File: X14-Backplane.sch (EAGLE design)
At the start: 34 parts, among them J2 PXC-PTSM-04-RA-1778641, J3 PXC-8-RA-1778683, J8 PXC-8-RA-1778683

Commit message: STEPS!
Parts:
- DIST_TO_BACKPLANE: device Samtec MPPT Hermaphoditic 10 pos - MPPT-10-01-01-L-RA-SD:MPPT-10-01-01-L-RA-SD -> CONN, Samtec MPPT Hermaphoditic 10 pos - MPPT-10-01-01-L-RA-SD:MPPT-10-01-01-L-RA-SD
- J2: device Phoenix Contact PTSM-04-V-1778573:PXC-PTSM-04-RA-1778641 -> CONN, Phoenix Contact PTSM-04-V-1778573:PXC-PTSM-04-RA-1778641
- J3, J8: device Phoenix Contact PTSM 8 pin:PXC-8-RA-1778683 -> CONN, Phoenix Contact PTSM 8 pin:PXC-8-RA-1778683
- U$1, U$2, U$3: device BLHeli_32 45A:BACKPLANE_CONNECTORSBKP -> Conn, Backplane-ESC-Controller:BACKPLANE_CONNECTORSBKP
- U$5, U$6, U$7: device Backplane_ESC_adapter:BACKPLANE_ESC_ADAPTER_PWRBKP -> CONN, Backplane_ESC_adapter:BACKPLANE_ESC_ADAPTER_PWRBKP
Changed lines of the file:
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@@
 <part name="FRAME2" library="SparkFun-Aesthetics" library_urn="urn:adsk.eagle:library:507" deviceset="FRAME-A4L" device=""/>
 <part name="MUX" library="BackplaneMUX" deviceset="TI-SN74LV4052A" device=""/>
-<part name="J2" library="Phoenix Contact PTSM-04-V-1778573" deviceset="PXC-PTSM-04-RA-1778641" device=""/>
-<part name="J3" library="Phoenix Contact PTSM 8 pin" deviceset="PXC-8-RA-1778683" device="" package3d_urn="urn:adsk.eagle:package:25224885/2"/>
+<part name="J2" library="CONN, Phoenix Contact PTSM-04-V-1778573" deviceset="PXC-PTSM-04-RA-1778641" device="" package3d_urn="urn:adsk.eagle:package:33723680/2"/>
+<part name="J3" library="CONN, Phoenix Contact PTSM 8 pin" deviceset="PXC-8-RA-1778683" device="" package3d_urn="urn:adsk.eagle:package:25224885/2"/>
 <part name="R4" library="SparkFun-Resistors" library_urn="urn:adsk.eagle:library:532" deviceset="26.7KOHM" device="0603-1/10W-1%" package3d_urn="urn:adsk.eagle:package:39650/1" value="22k"/>
 <part name="R1" library="SparkFun-Resistors" library_urn="urn:adsk.eagle:library:532" deviceset="10KOHM" device="-0603-1/10W-1%" package3d_urn="urn:adsk.eagle:package:39650/1" value="10k"/>
 <part name="R5" library="SparkFun-Resistors" library_urn="urn:adsk.eagle:library:532" deviceset="1KOHM" device="-0603-1/10W-1%" package3d_urn="urn:adsk.eagle:package:39650/1" value="4.7k"/>
-<part name="DIST_TO_BACKPLANE" library="Samtec MPPT Hermaphoditic 10 pos - MPPT-10-01-01-L-RA-SD" deviceset="MPPT-10-01-01-L-RA-SD" device="" package3d_urn="urn:adsk.eagle:package:25115828/2"/>
+<part name="DIST_TO_BACKPLANE" library="CONN, Samtec MPPT Hermaphoditic 10 pos - MPPT-10-01-01-L-RA-SD" deviceset="MPPT-10-01-01-L-RA-SD" device="" package3d_urn="urn:adsk.eagle:package:25115828/2"/>
 <part name="H1" library="Mounting Holes" deviceset="6-32-HOLE" device="" package3d_urn="urn:adsk.eagle:package:24384748/2"/>
 <part name="H2" library="Mounting Holes" deviceset="6-32-HOLE" device="" package3d_urn="urn:adsk.eagle:package:24384748/2"/>
-<part name="U$5" library="Backplane_ESC_adapter" deviceset="BACKPLANE_ESC_ADAPTER_PWR" device="BKP"/>
-<part name="U$6" library="Backplane_ESC_adapter" deviceset="BACKPLANE_ESC_ADAPTER_PWR" device="BKP"/>
-<part name="U$7" library="Backplane_ESC_adapter" deviceset="BACKPLANE_ESC_ADAPTER_PWR" device="BKP"/>
-<part name="U$1" library="BLHeli_32 45A" deviceset="BACKPLANE_CONNECTORS" device="BKP"/>
-<part name="U$2" library="BLHeli_32 45A" deviceset="BACKPLANE_CONNECTORS" device="BKP"/>
-<part name="U$3" library="BLHeli_32 45A" deviceset="BACKPLANE_CONNECTORS" device="BKP"/>
+<part name="U$5" library="CONN, Backplane_ESC_adapter" deviceset="BACKPLANE_ESC_ADAPTER_PWR" device="BKP" package3d_urn="urn:adsk.eagle:package:33723362/2" value="BACKPLANE_ESC_ADAPTER_PWRBKP"/>
+<part name="U$6" library="CONN, Backplane_ESC_adapter" deviceset="BACKPLANE_ESC_ADAPTER_PWR" device="BKP" package3d_urn="urn:adsk.eagle:package:33723362/2" value="BACKPLANE_ESC_ADAPTER_PWRBKP"/>
+<part name="U$7" library="CONN, Backplane_ESC_adapter" deviceset="BACKPLANE_ESC_ADAPTER_PWR" device="BKP" package3d_urn="urn:adsk.eagle:package:33723362/2" value="BACKPLANE_ESC_ADAPTER_PWRBKP"/>
+<part name="U$1" library="Conn, Backplane-ESC-Controller" deviceset="BACKPLANE_CONNECTORS" device="BKP" package3d_urn="urn:adsk.eagle:package:33721620/2"/>
+<part name="U$2" library="Conn, Backplane-ESC-Controller" deviceset="BACKPLANE_CONNECTORS" device="BKP" package3d_urn="urn:adsk.eagle:package:33721620/2"/>
+<part name="U$3" library="Conn, Backplane-ESC-Controller" deviceset="BACKPLANE_CONNECTORS" device="BKP" package3d_urn="urn:adsk.eagle:package:33721620/2"/>
 <part name="R7" library="SparkFun-Resistors" library_urn="urn:adsk.eagle:library:532" deviceset="68.1KOHM" device="-0603-1/10W-1%" package3d_urn="urn:adsk.eagle:package:39650/1" value="60"/>
 <part name="R8" library="SparkFun-Resistors" library_urn="urn:adsk.eagle:library:532" deviceset="68.1KOHM" device="-0603-1/10W-1%" package3d_urn="urn:adsk.eagle:package:39650/1" value="60"/>
@@
 <part name="U$8" library="OTHER, Push button - FSM2JMTR" deviceset="DISCRETECOMPONENTS_SWITCH" device="" package3d_urn="urn:adsk.eagle:package:24384574/2"/>
 <part name="R9" library="SparkFun-Resistors" library_urn="urn:adsk.eagle:library:532" deviceset="10KOHM" device="-0603-1/10W-1%" package3d_urn="urn:adsk.eagle:package:39650/1" value="10k"/>
-<part name="U$4" library="CONN, Distribution-Backplane" deviceset="BACKPLANE-DISTRIBUTION" device=""/>
-<part name="J8" library="Phoenix Contact PTSM 8 pin" deviceset="PXC-8-RA-1778683" device="" package3d_urn="urn:adsk.eagle:package:25224885/2"/>
-<part name="U$9" library="PI-SHIELD, Solenoid-Backplane" deviceset="7X_CONN" device=""/>
-<part name="U$10" library="CONN, DataConversion-Backplane Connector- SAMTEC CLT-107-01-F-D" deviceset="BACKPLANE-&gt;DATACONV" device=""/>
+<part name="U$4" library="CONN, Distribution-Backplane" deviceset="BACKPLANE-DISTRIBUTION" device="" package3d_urn="urn:adsk.eagle:package:32878650/2"/>
+<part name="J8" library="CONN, Phoenix Contact PTSM 8 pin" deviceset="PXC-8-RA-1778683" device="" package3d_urn="urn:adsk.eagle:package:25224885/2"/>
+<part name="U$9" library="PI-SHIELD, Solenoid-Backplane" deviceset="7X_CONN" device="" package3d_urn="urn:adsk.eagle:package:33723615/2"/>
+<part name="U$10" library="CONN, DataConversion-Backplane Connector- SAMTEC CLT-107-01-F-D" deviceset="BACKPLANE-&gt;DATACONV" device="" package3d_urn="urn:adsk.eagle:package:33723582/2"/>
 <part name="C1" library="CAP, aluminin-capacitor-brick-UCM1H331MNL1GS" deviceset="UCM1H331MNL1GS" device="" package3d_urn="urn:adsk.eagle:package:24202090/2" value="330uF"/>
 <part name="C2" library="CAP, aluminin-capacitor-brick-UCM1H331MNL1GS" deviceset="UCM1H331MNL1GS" device="" package3d_urn="urn:adsk.eagle:package:24202090/2" value="330uF"/>

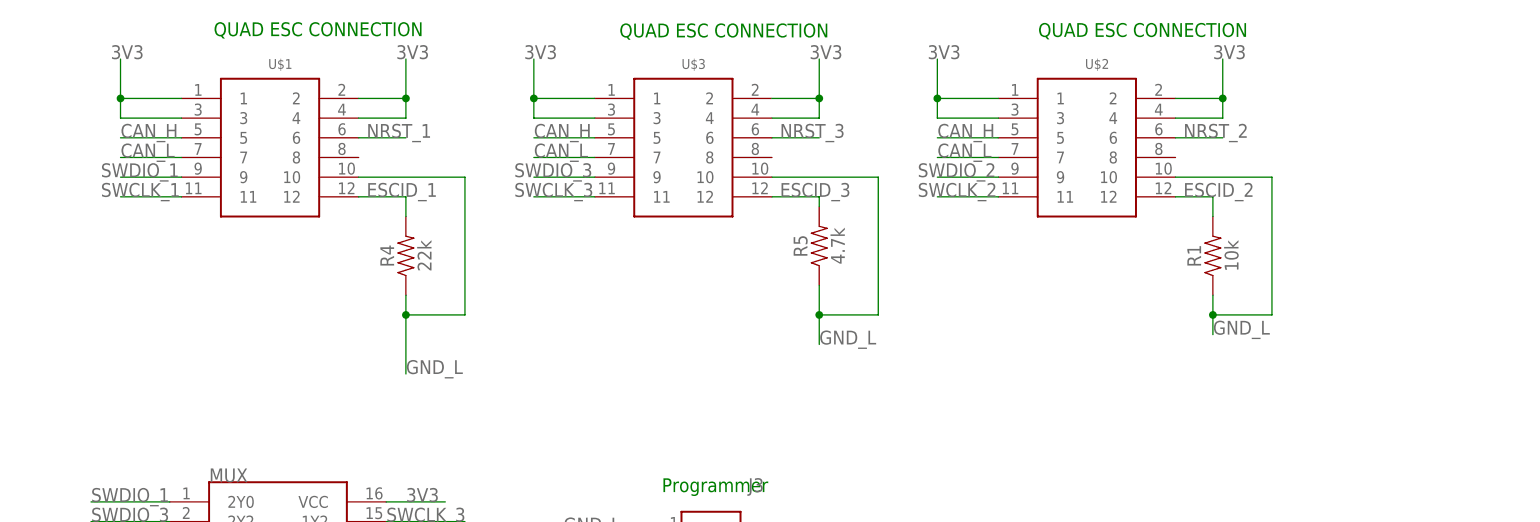
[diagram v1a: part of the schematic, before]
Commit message: new connector UwU SQT
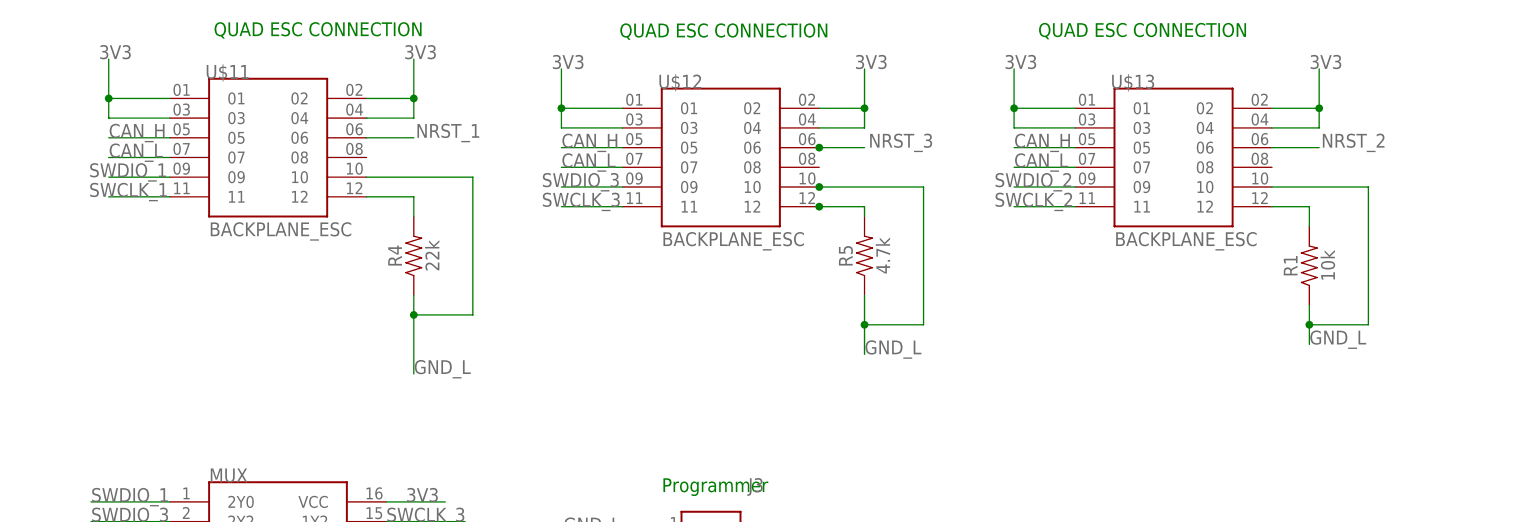
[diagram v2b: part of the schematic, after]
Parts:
- removed U$1, U$2, U$3: BACKPLANE_CONNECTORSBKP, Conn, Backplane-ESC-Controller:BACKPLANE_CONNECTORSBKP
- added U$11, U$12, U$13: BACKPLANE_ESC, SQT-106-01-F-D:BACKPLANE_ESC
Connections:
- net 3V3: now also U$11.01, U$11.02, U$11.03, U$11.04, U$12.01, U$12.02, U$12.03, U$12.04, U$13.01, U$13.02, U$13.03, U$13.04; no longer U$1.1, U$1.2, U$1.3, U$1.4, U$2.1, U$2.2, U$2.3, U$2.4, U$3.1, U$3.2, U$3.3, U$3.4
- net CAN_H: now also U$11.05, U$12.05, U$13.05; no longer U$1.5, U$2.5, U$3.5
- net CAN_L: now also U$11.07, U$12.07, U$13.07; no longer U$1.7, U$2.7, U$3.7
- net ESCID_1: now also U$11.12; no longer U$1.12
- net ESCID_2: now also U$13.12; no longer U$2.12
- net ESCID_3: now also U$12.12; no longer U$3.12
- net GND_L: now also U$11.10, U$12.10, U$13.10; no longer U$1.10, U$2.10, U$3.10
- net NRST_1: now also U$11.06; no longer U$1.6
- net NRST_2: now also U$13.06; no longer U$2.6
- net NRST_3: now also U$12.06; no longer U$3.6
- net SWCLK_1: now also U$11.11; no longer U$1.11
- net SWCLK_2: now also U$13.11; no longer U$2.11
- net SWCLK_3: now also U$12.11; no longer U$3.11
- net SWDIO_1: now also U$11.09; no longer U$1.9
- net SWDIO_2: now also U$13.09; no longer U$2.9
- net SWDIO_3: now also U$12.09; no longer U$3.9
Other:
- moved on the sheet: R1, R4, R5
